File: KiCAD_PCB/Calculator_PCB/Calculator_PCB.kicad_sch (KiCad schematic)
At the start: 108 parts, among them J1 USB_B_Micro, SW1 +, SW10 E, SW11 D, SW12 C, SW13 *, SW14 R, SW15 F, SW16 V, SW17 =, SW18 T, SW19 G, SW2 Q, SW20 B, SW21 SQRT, SW22 Y, SW23 H, SW24 N, SW25 e^x (ln), SW26 U, SW27 J, SW28 M, SW29 10^x (log), SW3 A, SW30 I, SW31 K, SW32 [ ] ({ }), SW33 Symbol's, SW34 O, SW35 L, SW36 ; (:), SW37 Menu, SW38 P, SW39 Trig, SW4 Z, SW40 Greek, SW5 -, SW6 W, SW7 S, SW8 X, SW9 /, U1 W25Q128JVS, U2 RP2040, U3 NCP1117-3.3_SOT223, Y1 ABLS-12.000MHZ-B4-T

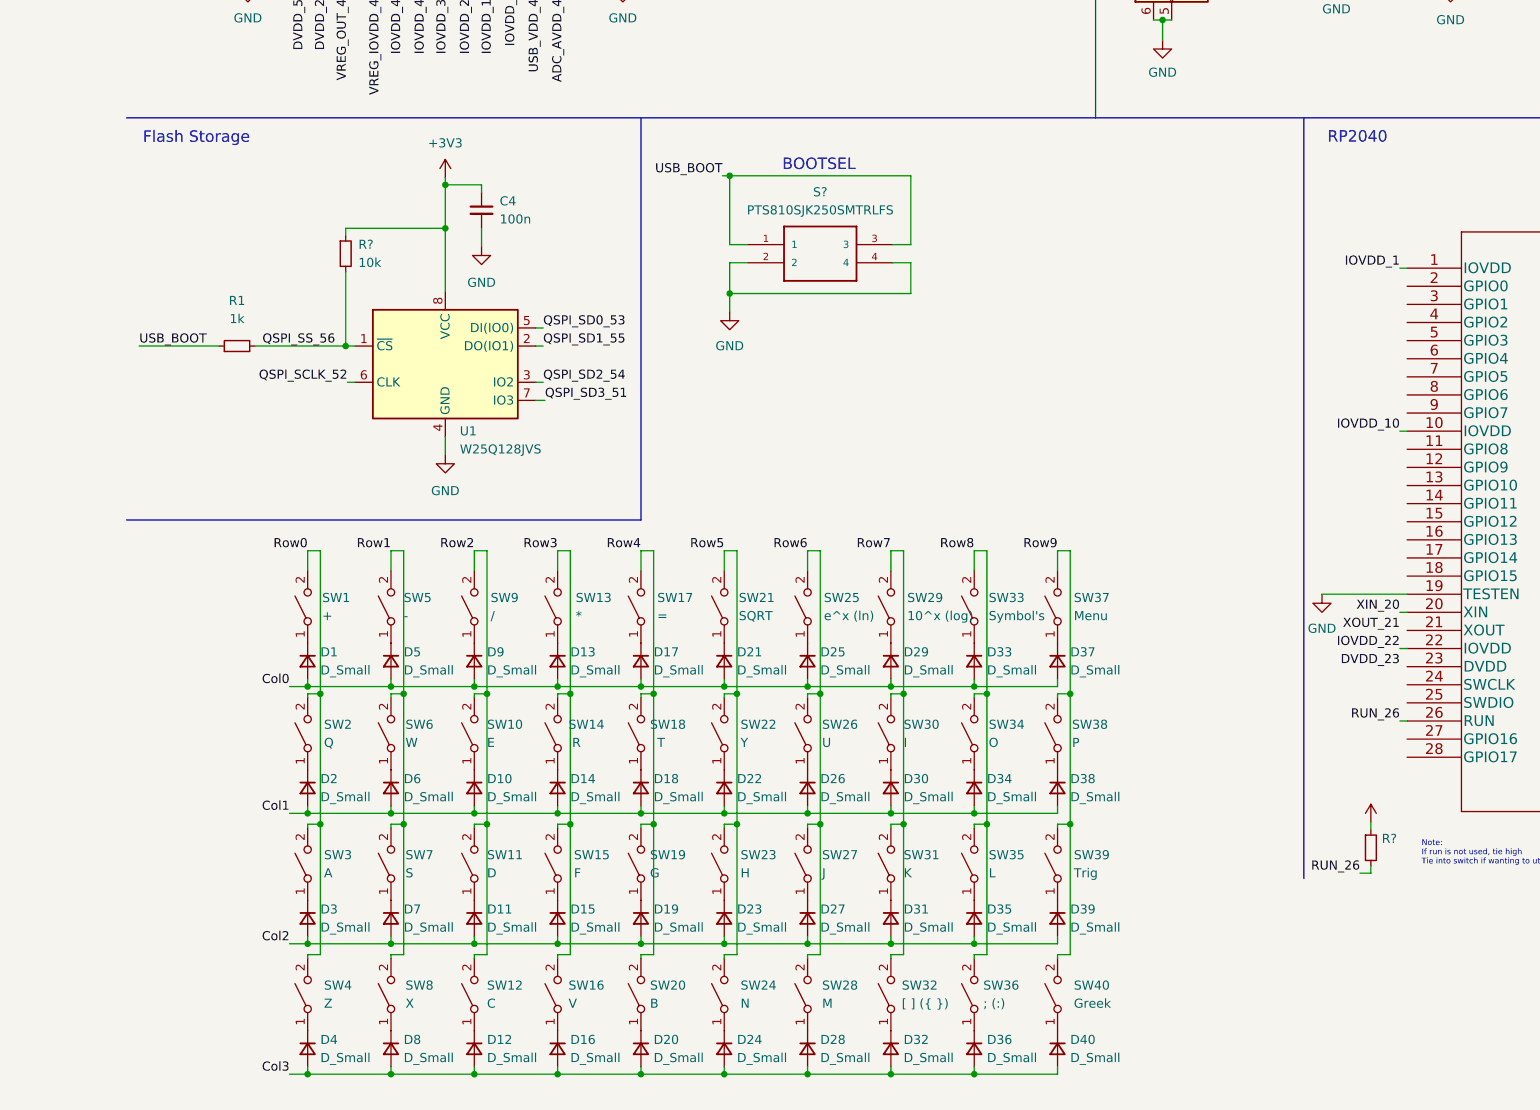
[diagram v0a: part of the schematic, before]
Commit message: PCB Updates
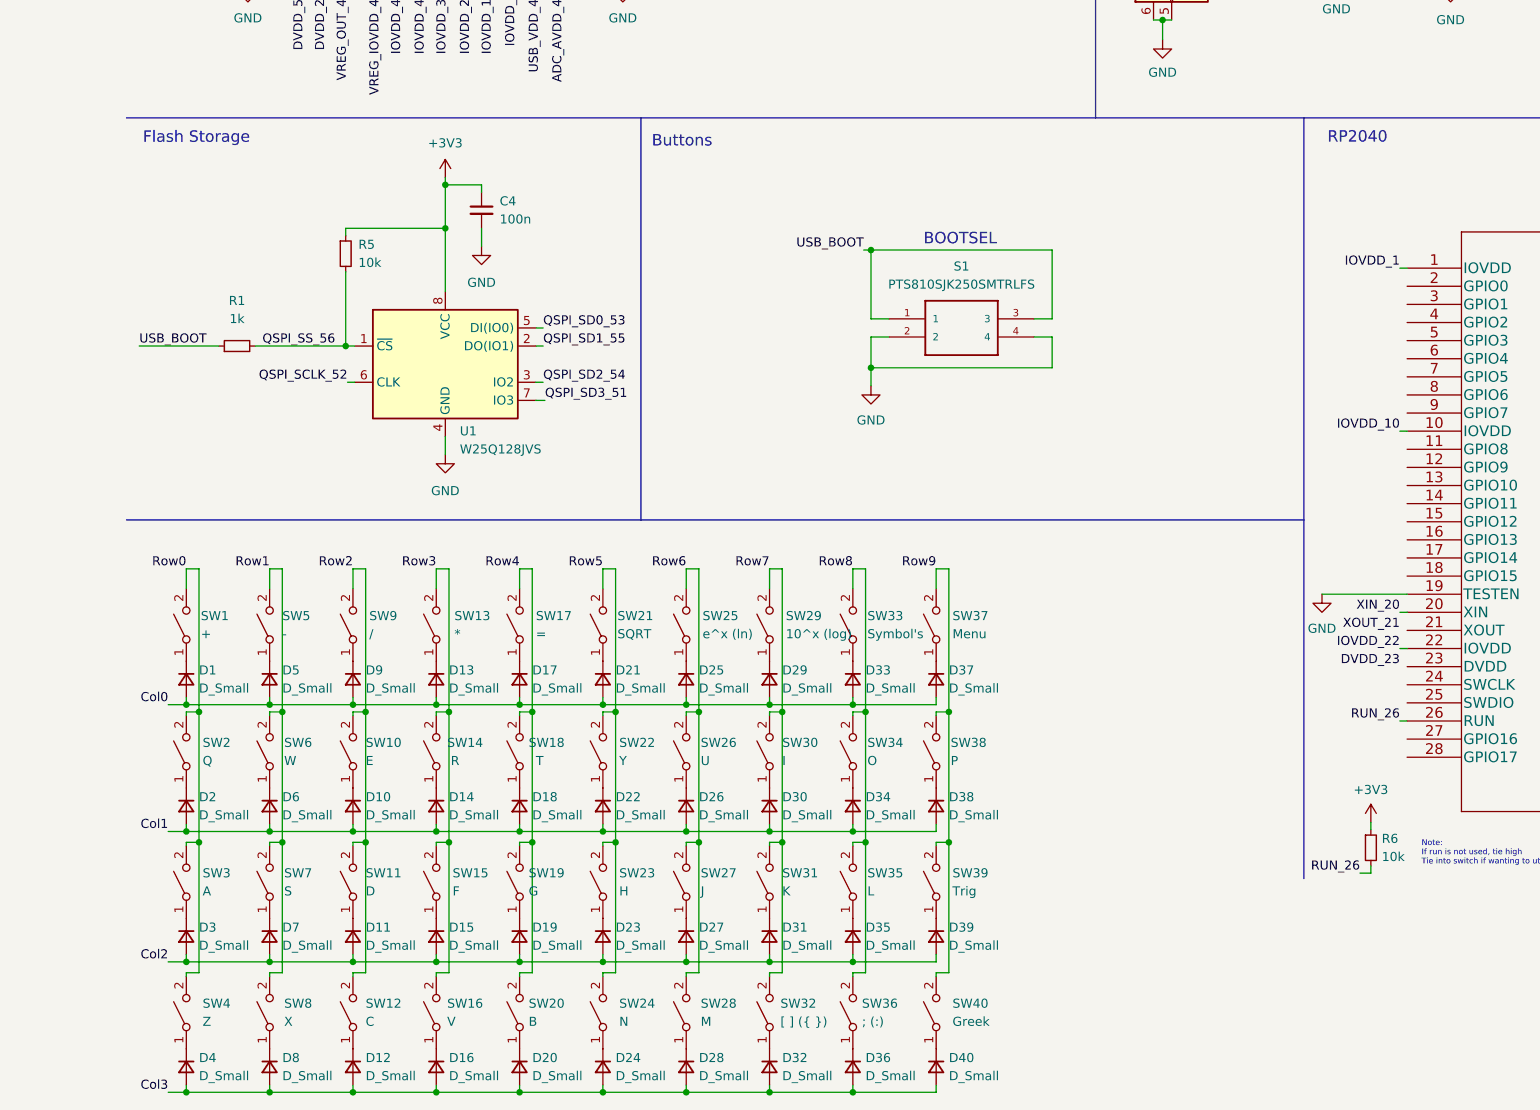
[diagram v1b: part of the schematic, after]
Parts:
- C1, C10, C11, C12, C13, C14, C15, C16, C2, C3, C4, C5, C6, C7, C8, C9: footprint (none) -> Capacitor_SMD:C_01005_0402Metric_Pad0.57x0.30mm_HandSolder
- D1, D10, D11, D12, D13, D14, D15, D16, D17, D18, D19, D2, D20, D21, D22, D23, D24, D25, D26, D27, D28, D29, D3, D30, D31, D32, D33, D34, D35, D36, D37, D38, D39, D4, D40, D5, D6, D7, D8, D9: footprint (none) -> Diode_SMD:D_0402_1005Metric_Pad0.77x0.64mm_HandSolder
- R6: renamed from R?; value (none) -> 10k
- S1: renamed from S?; footprint PTS810SJG250SMTRLFS -> (none)
- U2: footprint IC57_RP2040 -> (none)
- gave numbers to parts that had none: 1
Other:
- note added: "Buttons"
- moved on the sheet: D1, D10, D11, D12, D13, D14, D15, D16, D17, D18, D19, D2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
